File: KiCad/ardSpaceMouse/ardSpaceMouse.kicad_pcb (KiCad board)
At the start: 2 copper layers, 60.3 x 38.1 mm, 5 parts, among them SW1 SW_Push, SW2 SW_Push, SW3 SW_Push, U1 Sparkfun_Pro_Micro, U2 JOYSTICKPTH_my

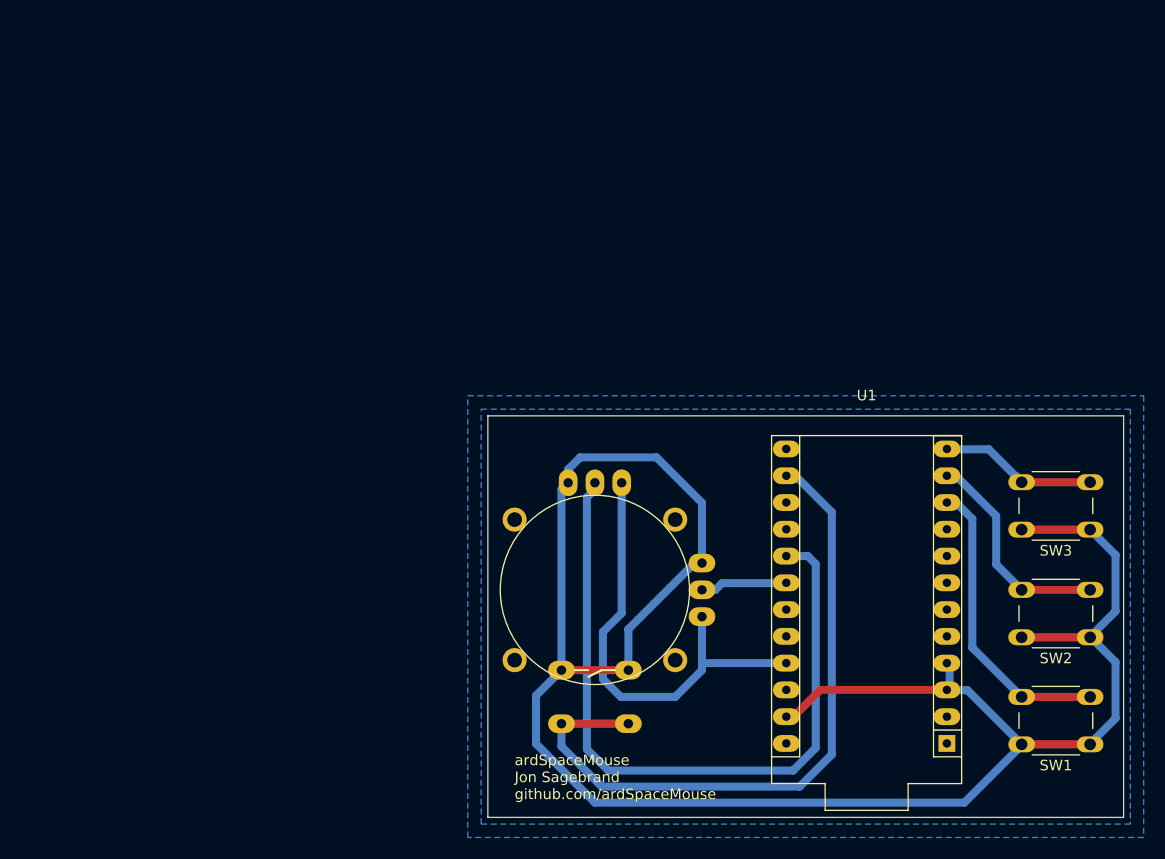
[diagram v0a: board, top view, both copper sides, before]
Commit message: scad updates
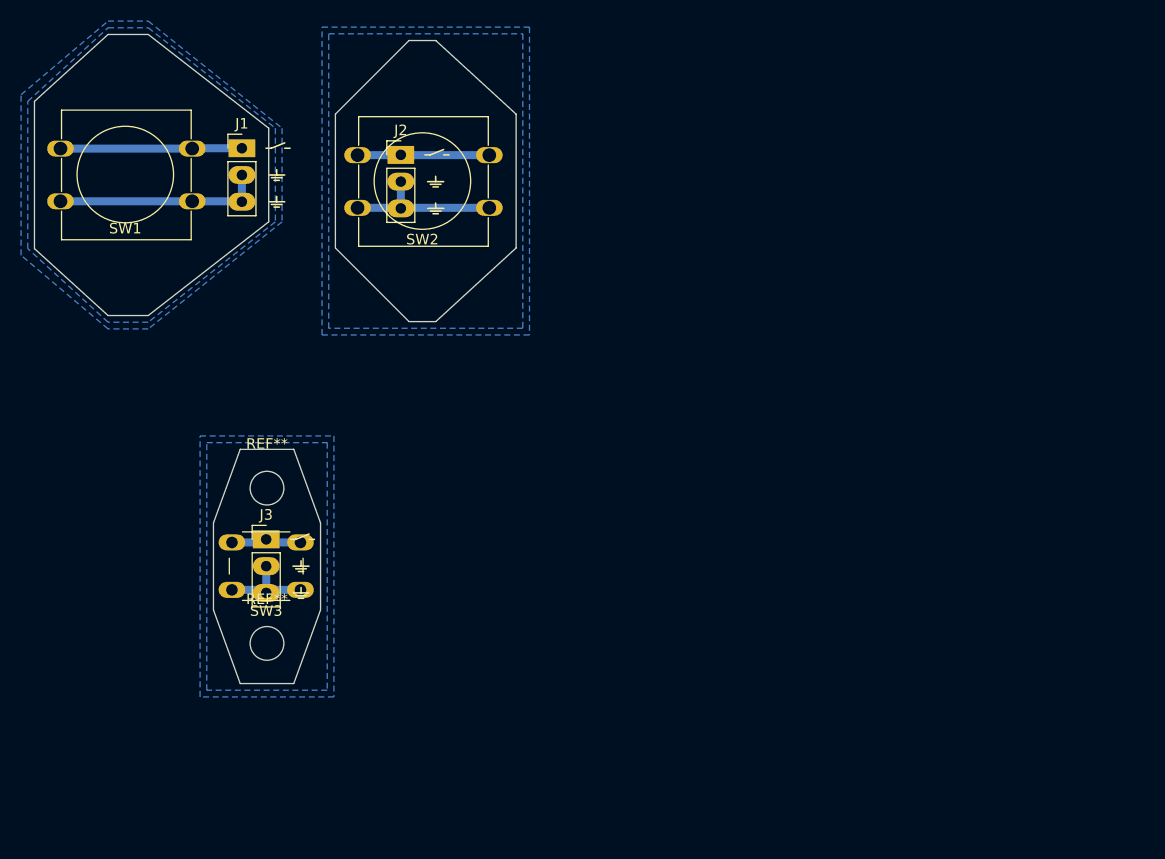
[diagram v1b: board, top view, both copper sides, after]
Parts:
- removed U1: Sparkfun_Pro_Micro, My_Arduino2:Sparkfun_Pro_Micro_large
- removed U2: JOYSTICKPTH_my, SparkFun_Electromechanical:JOYSTICK_large
- added J1: 3-pin_button+2xGND_header, My_Headers:3-pin_button+2xGND_header_large, F.Cu at (71.3, 42.5)
- added J2: 3-pin_button+2xGND_header, My_Headers:3-pin_button+2xGND_header_large, F.Cu at (86.4, 43.2)
- added J3: 3-pin_button+2xGND_header, My_Headers:3-pin_button+2xGND_header_large, F.Cu at (73.6, 79.7)
- added REF**: MountingHole_3.2mm_M3, MountingHole:MountingHole_3.2mm_M3, F.Cu at (73.7, 74.8)
- added REF**: MountingHole_3.2mm_M3, MountingHole:MountingHole_3.2mm_M3, F.Cu at (73.7, 89.5)
- SW1, SW2: footprint My_Misc:SW_PUSH_6mm_large -> My_Misc:SW_PUSH-12mm_large
- moved SW1 99.6 mm to (66.6, 47.6)
- moved SW3 75.1 mm to (76.8, 84.5)
- moved SW2 70.1 mm to (94.8, 48.2)
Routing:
- net GND: track 189.8 -> 43.9 mm
- net X: track 69.6 -> 0.00 mm
- net Net-(U1-Pad14): track 66.1 -> 0.00 mm
- net VCC: track 43.6 -> 0.00 mm
- net Net-(J1-Pad1): track 28.8 -> 17.2 mm
- net Net-(J3-Pad1): track 16.0 -> 6.37 mm
- net Net-(J2-Pad1): track 21.1 -> 12.5 mm
- net Y: track 8.52 -> 0.00 mm
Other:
- board size 60.3 x 38.1 mm -> 45.7 x 61.6 mm
- board text removed: "ardSpaceMouse Jon Sagebrand github.com/ardSpaceMouse"
